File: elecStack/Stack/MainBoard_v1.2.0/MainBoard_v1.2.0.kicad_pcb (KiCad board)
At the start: 2 copper layers, 126.5 x 101.5 mm, 62 parts, among them J1 Conn_01x04_Socket, J2 Conn_01x06_Pin, J3 Conn_01x06_Pin, J4 Conn_01x07_Socket, J5 Conn_01x07_Socket, J6 Conn_01x04_Socket, Q1 NMOS, SW1 SW_Push, SW2 SW_Wuerth_450301014042, U1 RASPBERRY_PI_PICO

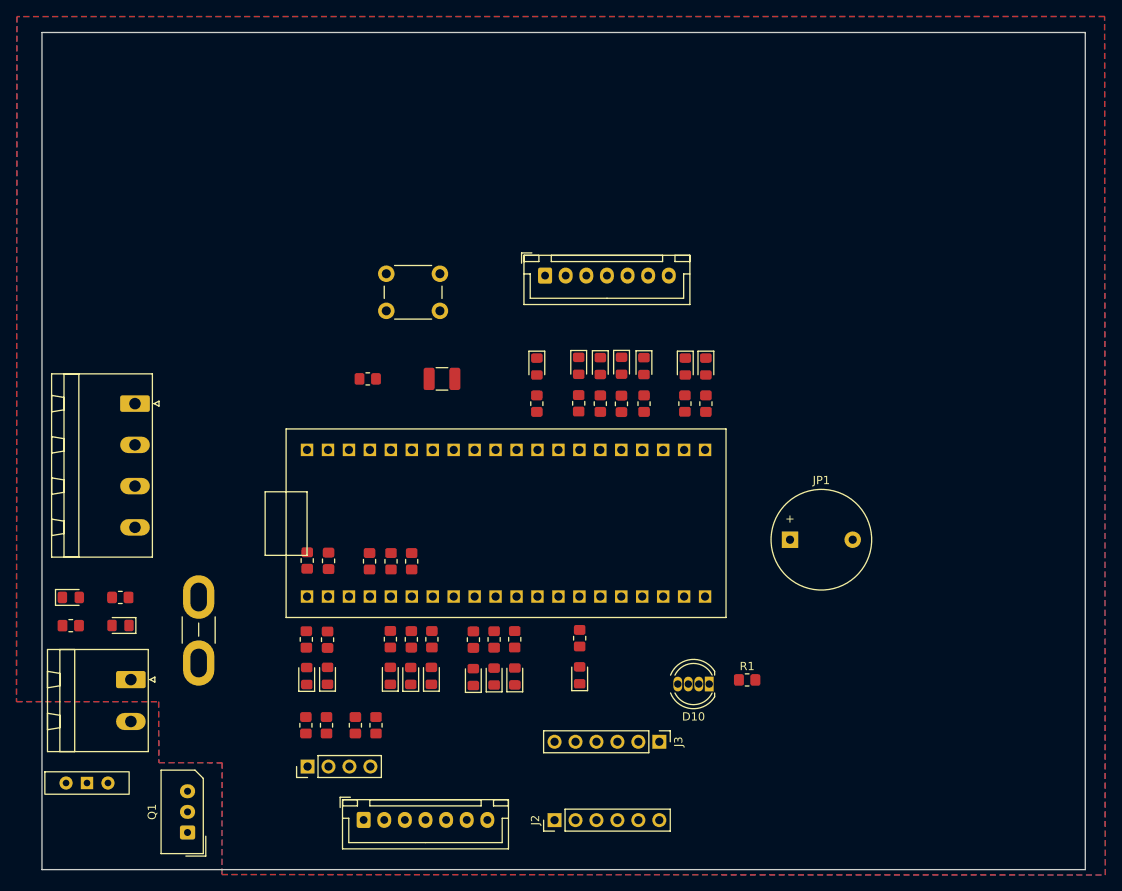
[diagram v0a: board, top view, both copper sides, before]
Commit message: routing done
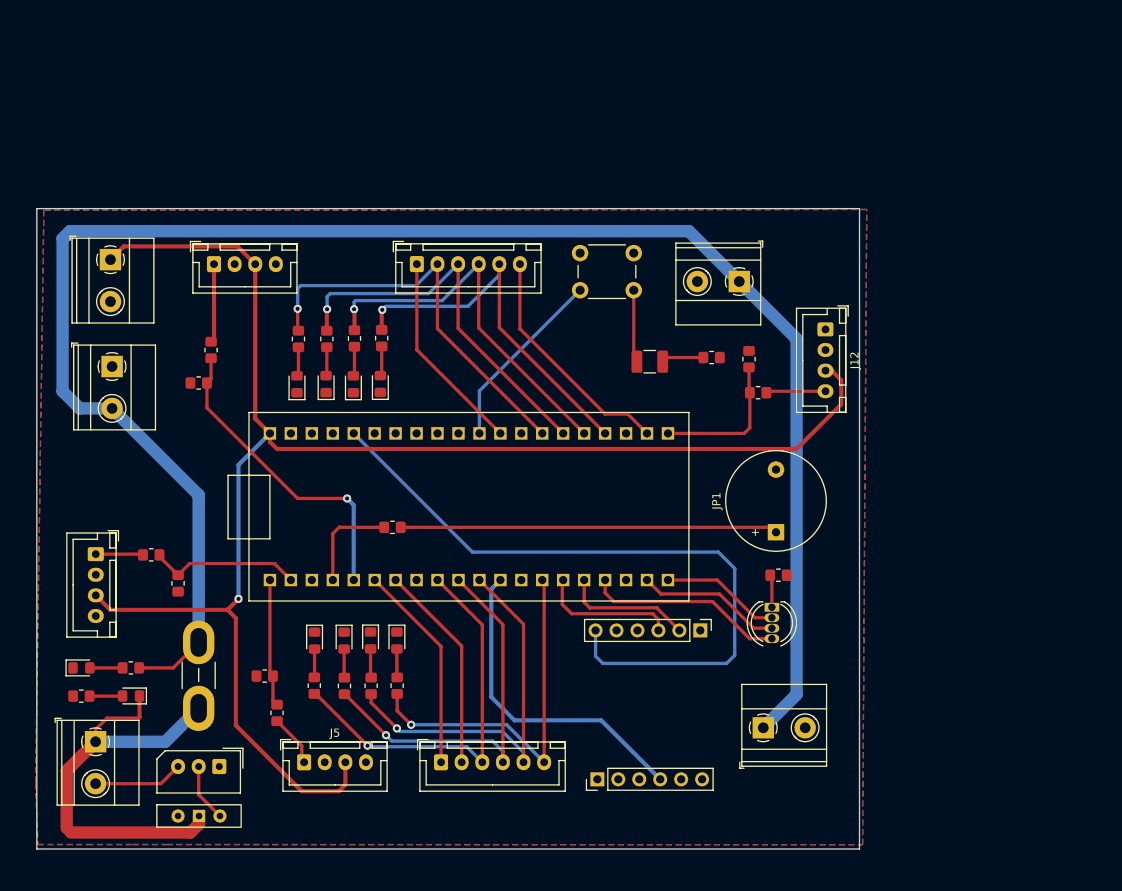
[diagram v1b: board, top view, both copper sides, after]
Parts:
- removed D1, D15, D16, D17, D18, D19, D8, D9: GREEN_LED, LED_SMD:LED_0805_2012Metric_Pad1.15x1.40mm_HandSolder
- removed J1: Conn_01x04_Socket, Connector_Phoenix_MSTB:PhoenixContact_MSTBA_2,5_4-G_1x04_P5.00mm_Horizontal
- removed J6: Conn_01x04_Socket, Connector_PinHeader_2.54mm:PinHeader_1x04_P2.54mm_Vertical
- removed R11, R17, R20, R21, R22, R24, R3, R6: 150, Resistor_SMD:R_0805_2012Metric_Pad1.20x1.40mm_HandSolder
- added BATTERY_CONN2: Conn_01x02_Socket, TerminalBlock_Phoenix:TerminalBlock_Phoenix_MKDS-1,5-2-5.08_1x02_P5.08mm_Horizontal, F.Cu at (59.8, 94.5)
- added BATTERY_CONN3: Conn_01x02_Socket, TerminalBlock_Phoenix:TerminalBlock_Phoenix_MKDS-1,5-2-5.08_1x02_P5.08mm_Horizontal, F.Cu at (60.0, 107.5)
- added J10: Conn_01x04_Socket, Connector_JST:JST_XH_B4B-XH-A_1x04_P2.50mm_Vertical, F.Cu at (58.0, 130.2)
- added J11: Conn_01x04_Socket, Connector_JST:JST_XH_B4B-XH-A_1x04_P2.50mm_Vertical, F.Cu at (72.4, 95.1)
- added J12: Conn_01x04_Socket, Connector_JST:JST_XH_B4B-XH-A_1x04_P2.50mm_Vertical, F.Cu at (146.5, 103.0)
- added J7: Conn_01x06_Socket, Connector_JST:JST_XH_B6B-XH-A_1x06_P2.50mm_Vertical, F.Cu at (97.0, 95.1)
- added J8: Conn_01x02_Pin, TerminalBlock_Phoenix:TerminalBlock_Phoenix_MKDS-1,5-2-5.08_1x02_P5.08mm_Horizontal, F.Cu at (136.0, 97.2)
- added J9: Conn_01x02_Pin, TerminalBlock_Phoenix:TerminalBlock_Phoenix_MKDS-1,5-2-5.08_1x02_P5.08mm_Horizontal, F.Cu at (139.0, 151.3)
- BATTERY_CONN1: footprint Connector_Phoenix_MSTB:PhoenixContact_MSTBA_2,5_2-G-5,08_1x02_P5.08mm_Horizontal -> TerminalBlock_Phoenix:TerminalBlock_Phoenix_MKDS-1,5-2-5.08_1x02_P5.08mm_Horizontal
- J4: value Conn_01x07_Socket -> Conn_01x06_Socket; footprint Connector_JST:JST_XH_B7B-XH-A_1x07_P2.50mm_Vertical -> Connector_JST:JST_XH_B6B-XH-A_1x06_P2.50mm_Vertical
- J5: value Conn_01x07_Socket -> Conn_01x04_Socket; footprint Connector_JST:JST_XH_B7B-XH-A_1x07_P2.50mm_Vertical -> Connector_JST:JST_XH_B4B-XH-A_1x04_P2.50mm_Vertical
- moved R31 61.4 mm to (138.3, 110.7), turned to 180 degrees
- moved J4 60.3 mm to (99.9, 155.5)
- moved R27 48.7 mm to (72.0, 105.5), turned to -90 degrees
- moved R33 47.7 mm to (137.2, 106.6)
- moved R13 41.8 mm to (132.7, 106.4), turned to 180 degrees
- moved R7 34.9 mm to (82.6, 104.2), turned to -90 degrees
- moved D4 34.2 mm to (82.4, 109.7), turned to 90 degrees
- moved R8 34.1 mm to (86.0, 104.2), turned to -90 degrees
- moved R9 33.3 mm to (89.4, 104.1), turned to -90 degrees
- moved D5 33.3 mm to (85.9, 109.6), turned to 90 degrees
- moved R10 32.8 mm to (92.7, 104.1), turned to -90 degrees
- moved D6 32.6 mm to (89.3, 109.7), turned to 90 degrees
- moved D7 32.0 mm to (92.5, 109.6), turned to 90 degrees
- moved R29 31.8 mm to (70.5, 109.5), turned to 180 degrees
- moved R23 29.6 mm to (64.7, 130.3), turned to 0 degrees
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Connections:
- J3 pad 5: 3V -> unconnected-(J3-Pin_5-Pad5)
- J4 pad 1: PWR_IN -> EN_3
- J4 pad 2: EN_1 -> EN_4
- J4 pad 3: IN_1_1 -> IN_1_3
- J4 pad 4: IN_2_1 -> IN_2_3
- J4 pad 5: IN_1_2 -> IN_1_4
- J4 pad 6: IN_2_2 -> IN_2_4
- J5 pad 1: PWR_IN -> ENC_A_1
- J5 pad 2: EN_3 -> ENC_B_1
- J5 pad 3: IN_1_3 -> 5V_buck
- J5 pad 4: IN_2_3 -> GND
- U1 pad GP16: EN_4 -> ENC_A_4_3.3
- U1 pad GP28_A2: V_measure -> unconnected-(U1-PadGP28_A2)
- U1 pad GP4: ENC_A_4_3.3 -> EN_3
- U1 pad GP5: EN_3 -> EN_4
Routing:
- net PWR_IN: track 0.00 -> 210.2 mm
- net 5V_buck: track 0.00 -> 192.9 mm, vias 0 -> 1
- net 3V3: track 0.00 -> 84.3 mm
- net 12_V_battery: track 0.00 -> 53.8 mm
- net IN_1_1: track 0.00 -> 49.1 mm, vias 0 -> 1
- net IN_1_3: track 0.00 -> 48.1 mm, vias 0 -> 1
- net IN_2_3: track 0.00 -> 47.7 mm, vias 0 -> 1
- net IN_1_4: track 0.00 -> 47.5 mm, vias 0 -> 1
- net IN_2_1: track 0.00 -> 47.5 mm, vias 0 -> 1
- net IN_1_2: track 0.00 -> 46.3 mm, vias 0 -> 1
- net Net-(JP1-A): track 0.00 -> 45.7 mm
- net IN_2_2: track 0.00 -> 45.6 mm, vias 0 -> 1
- net IN_2_4: track 0.00 -> 44.9 mm, vias 0 -> 1
- net RST: track 0.00 -> 39.3 mm
- net ENC_A_3_3.3: track 0.00 -> 38.0 mm, vias 0 -> 1
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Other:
- board size 126.5 x 101.5 mm -> 99.8 x 77.6 mm
